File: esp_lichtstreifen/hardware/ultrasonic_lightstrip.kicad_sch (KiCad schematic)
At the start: 8 parts, among them J1 Barrel_Jack_Switch, J2 HC-SR04, J3 WS2812B, J4 OLED, U1 ESP32-DevKitC

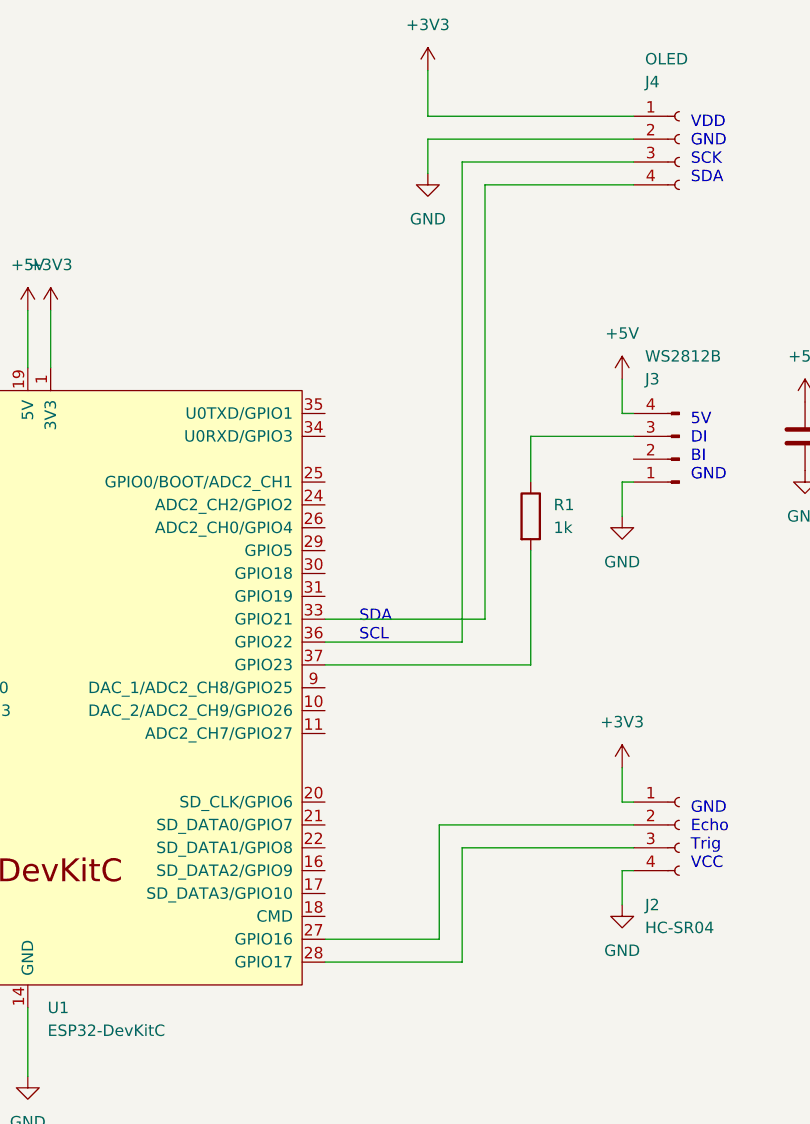
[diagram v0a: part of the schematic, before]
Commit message: finished first revision of PCB
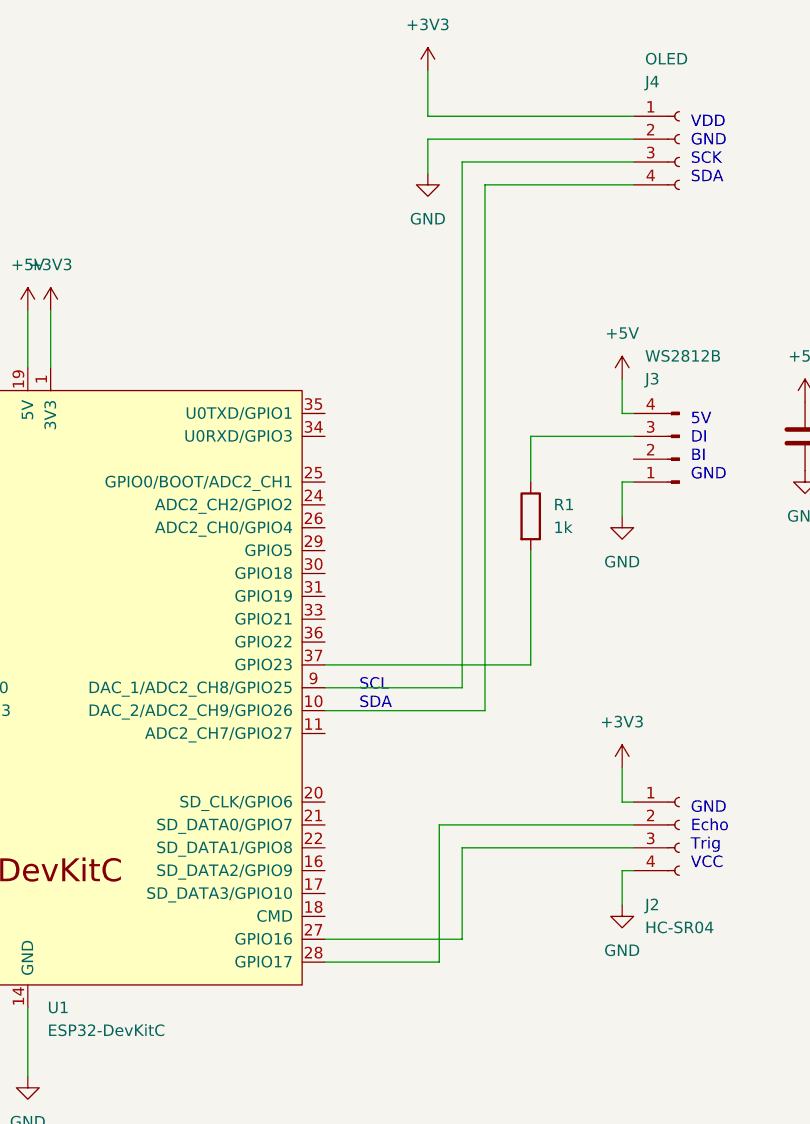
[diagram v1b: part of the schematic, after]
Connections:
- net at U1.10 (DAC_2/ADC2_CH9/GPIO26): now also J4.4 (Pin_4)
- net at U1.27 (GPIO16): now also J2.3 (Pin_3); no longer J2.2 (Pin_2)
- net at U1.28 (GPIO17): now also J2.2 (Pin_2); no longer J2.3 (Pin_3)
- net at U1.33 (GPIO21): no longer J4.4 (Pin_4)
- net at U1.36 (GPIO22): no longer J4.3 (Pin_3)
- net at U1.9 (DAC_1/ADC2_CH8/GPIO25): now also J4.3 (Pin_3)
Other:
- note added: "SCL SDA"
- note removed: "SDA SCL"
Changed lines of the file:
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@@
   (junction (at 54.61 44.45) (diameter 0) (color 0 0 0 0)
   )
-  (wire (pts (xy 190.5 127) (xy 175.26 127))
+  (wire (pts (xy 190.5 124.46) (xy 175.26 124.46))
     (stroke (width 0) (type default))
   )
@@
     (stroke (width 0) (type default))
   )
-  (wire (pts (xy 190.5 114.3) (xy 190.5 127))
+  (wire (pts (xy 190.5 114.3) (xy 190.5 124.46))
     (stroke (width 0) (type default))
   )
@@
     (stroke (width 0) (type default))
   )
-  (wire (pts (xy 175.26 91.44) (xy 190.5 91.44))
+  (wire (pts (xy 175.26 96.52) (xy 190.5 96.52))
     (stroke (width 0) (type default))
   )
@@
     (stroke (width 0) (type default))
   )
-  (wire (pts (xy 175.26 124.46) (xy 187.96 124.46))
+  (wire (pts (xy 175.26 127) (xy 187.96 127))
     (stroke (width 0) (type default))
   )
-  (wire (pts (xy 175.26 88.9) (xy 193.04 88.9))
+  (wire (pts (xy 175.26 99.06) (xy 193.04 99.06))
     (stroke (width 0) (type default))
   )
@@
     (stroke (width 0) (type default))
   )
+  (wire (pts (xy 193.04 40.64) (xy 193.04 99.06))
+    (stroke (width 0) (type default))
+  )
   (wire (pts (xy 48.26 41.91) (xy 54.61 41.91))
     (stroke (width 0) (type default))
@@
     (stroke (width 0) (type default))
   )
+  (wire (pts (xy 190.5 38.1) (xy 190.5 96.52))
+    (stroke (width 0) (type default))
+  )
   (wire (pts (xy 209.55 35.56) (xy 186.69 35.56))
     (stroke (width 0) (type default))
@@
     (stroke (width 0) (type default))
   )
-  (wire (pts (xy 187.96 124.46) (xy 187.96 111.76))
+  (wire (pts (xy 187.96 127) (xy 187.96 111.76))
     (stroke (width 0) (type default))
   )
@@
     (stroke (width 0) (type default))
   )
-  (wire (pts (xy 193.04 88.9) (xy 193.04 40.64))
-    (stroke (width 0) (type default))
-  )
   (wire (pts (xy 208.28 120.65) (xy 208.28 116.84))
-    (stroke (width 0) (type default))
-  )
-  (wire (pts (xy 190.5 91.44) (xy 190.5 38.1))
     (stroke (width 0) (type default))
   )
@@
     (effects (font (size 1.27 1.27)) (justify left bottom))
   )
-  (text "SDA\nSCL" (at 179.07 91.44 0)
+  (text "SCL\nSDA" (at 179.07 99.06 0)
     (effects (font (size 1.27 1.27)) (justify left bottom))
   )
